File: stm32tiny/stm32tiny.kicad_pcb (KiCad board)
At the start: 2 copper layers, 25.2 x 17.8 mm, 30 parts, among them J1 Conn_01x08, J2 Conn_01x07, J3 Conn_01x03, J4 USB_C_Receptacle_USB2.0, SW1 SW_Push, U1 STM32F042K6Tx, U2 AP7333

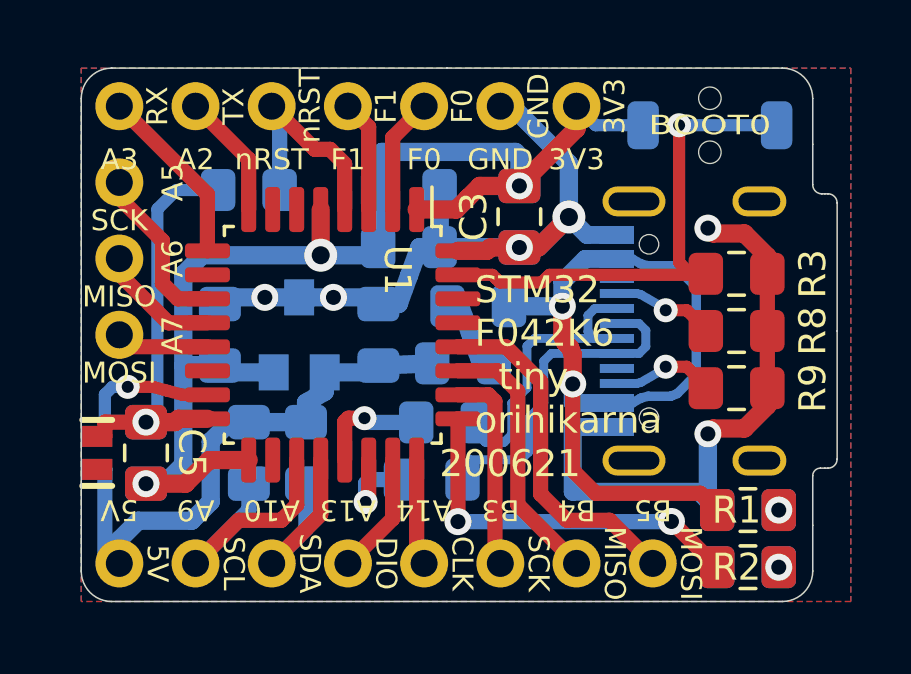
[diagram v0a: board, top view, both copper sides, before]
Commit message: 200904 for submit
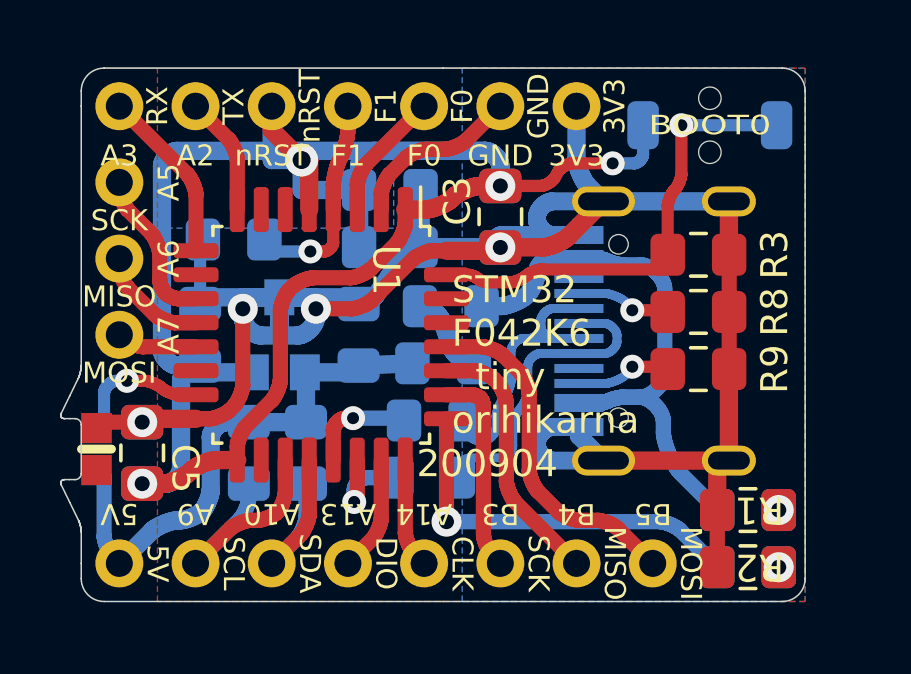
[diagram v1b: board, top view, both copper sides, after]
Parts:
- R1: value 1K -> 1K5
- R2: value 1K -> 330
- moved C9 1.73 mm to (5.08, 5.71)
- moved R3 1.42 mm to (20.6, 6.22)
- moved R8 1.42 mm to (20.6, 8.13)
- moved R9 1.42 mm to (20.6, 10.0)
- moved J4 1.02 mm to (21.6, 8.76)
- moved F1 0.91 mm to (12.3, 7.94)
- moved C1 0.66 mm to (9.25, 8.89)
- moved L1 0.66 mm to (12.1, 9.84)
- moved U2 0.66 mm to (6.60, 9.04)
- moved C2 0.66 mm to (3.96, 8.89)
- moved C3 0.63 mm to (14.0, 4.95)
- moved C4 0.63 mm to (14.0, 4.95)
- moved C7 0.63 mm to (10.3, 5.97)
- moved C8 0.63 mm to (10.3, 4.06)
- moved R6 0.41 mm to (11.8, 11.7)
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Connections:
- D1 pad 1: GND -> Net-(D1-Pad1)
- D1 pad 2: Net-(D1-Pad2) -> VBUS
- D2 pad 1: GND -> Net-(D2-Pad1)
- D2 pad 2: Net-(D2-Pad2) -> PA15
- J2 pad 3: NRST -> VCC
- J2 pad 4: PF1 -> NRST
- J2 pad 5: PF0 -> PF1
- J2 pad 6: GND -> PF0
- J2 pad 7: VCC -> GND
- J4 pad S1: Net-(J4-PadS1) -> GND
- R1 pad 1: VBUS -> Net-(D1-Pad1)
- R1 pad 2: Net-(D1-Pad2) -> GND
- R2 pad 1: PA15 -> Net-(D2-Pad1)
- R2 pad 2: Net-(D2-Pad2) -> GND
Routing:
- net VCC: track 43.2 -> 70.5 mm, vias 3 -> 4
- net GND: track 64.3 -> 83.1 mm, vias 7 -> 4
- net VBUS: track 26.7 -> 20.5 mm, vias 2 -> 0
- net Net-(J4-PadA7): track 10.7 -> 14.2 mm
- net BOOT0: track 17.5 -> 15.5 mm
- net PF0: track 3.88 -> 5.77 mm
- net 5V: track 19.5 -> 18.2 mm
- net Net-(J4-PadA6): track 11.3 -> 10.4 mm
- net PA9: track 9.07 -> 8.48 mm
- net PF1: track 3.73 -> 4.32 mm
- net PA15: track 12.7 -> 13.0 mm, vias 2 -> 1
- net NRST: track 7.65 -> 7.47 mm, vias 0 -> 1
- net Net-(D2-Pad2): vias 1 -> 0
- net Net-(D2-Pad1): vias 0 -> 1
- net Net-(D1-Pad2): vias 1 -> 0
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- added copper zone on B.Cu, net VCC
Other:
- board size 25.2 x 17.8 mm -> 24.8 x 17.8 mm
- board text added: "STM32 F042K6 tiny orihikarna 200904"
- board text removed: "STM32 F042K6 tiny orihikarna 200621"
